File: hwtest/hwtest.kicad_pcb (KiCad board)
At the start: 2 copper layers, 103.3 x 65 mm, 299 parts, among them P1 RZM001P02T2L, P10 RZM001P02T2L, P11 RZM001P02T2L, P12 RZM001P02T2L, P13 RZM001P02T2L, P14 RZM001P02T2L, P15 RZM001P02T2L, P16 RZM001P02T2L, P17 RZM001P02T2L, P18 RZM001P02T2L, P19 RZM001P02T2L, P2 RZM001P02T2L, P20 RZM001P02T2L, P21 RZM001P02T2L, P22 RZM001P02T2L, P23 RZM001P02T2L, P24 RZM001P02T2L, P25 RZM001P02T2L, P26 RZM001P02T2L, P27 RZM001P02T2L, P28 RZM001P02T2L, P29 RZM001P02T2L, P3 RZM001P02T2L, P30 RZM001P02T2L, P31 RZM001P02T2L, P32 RZM001P02T2L, P33 RZM001P02T2L, P34 RZM001P02T2L, P35 RZM001P02T2L, P36 RZM001P02T2L, P37 RZM001P02T2L, P38 RZM001P02T2L, P39 RZM001P02T2L, P4 RZM001P02T2L, P40 RZM001P02T2L, P41 RZM001P02T2L, P42 RZM001P02T2L, P43 RZM001P02T2L, P44 RZM001P02T2L, P45 RZM001P02T2L, P46 RZM001P02T2L, P47 RZM001P02T2L, P48 RZM001P02T2L, P49 RZM001P02T2L, P5 RZM001P02T2L, P50 RZM001P02T2L, P51 RZM001P02T2L, P52 RZM001P02T2L, P53 RZM001P02T2L, P54 RZM001P02T2L, P55 RZM001P02T2L, P56 RZM001P02T2L, P57 RZM001P02T2L, P6 RZM001P02T2L, P7 RZM001P02T2L, P8 RZM001P02T2L, P9 RZM001P02T2L

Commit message: Tweak design.
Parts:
- N10, N11, N12, N13, N17, N18, N19, N28, N29, N9: value 2SK3541 -> NX7002BKMB315
- P10, P11, P12, P13, P17, P18, P19, P28, P29, P9: value RZM001P02T2L -> BSS84KNC
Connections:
- R30 pad 2: Net-(D13-A) -> GND
- R36 pad 2: Net-(D16-A) -> GND
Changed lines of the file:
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@@
 			)
 		)
-		(property "Value" "2SK3541"
+		(property "Value" "NX7002BKMB315"
 			(at 0 1.6 0)
 			(layer "User.3")
@@
 			(layers "F.Cu" "F.Mask" "F.Paste")
 			(roundrect_rratio 0.25)
-			(net 114 "Net-(D16-A)")
+			(net 4 "GND")
 			(pintype "passive")
 		)
@@
 			)
 		)
-		(property "Value" "RZM001P02T2L"
+		(property "Value" "BSS84KNC"
 			(at 0 1.6 0)
 			(layer "User.3")
@@
 			)
 		)
-		(property "Value" "2SK3541"
+		(property "Value" "NX7002BKMB315"
 			(at 0 1.6 0)
 			(layer "User.3")
@@
 			)
 		)
-		(property "Value" "2SK3541"
+		(property "Value" "NX7002BKMB315"
 			(at 0 1.6 0)
 			(layer "User.3")
@@
 			)
 		)
-		(property "Value" "2SK3541"
+		(property "Value" "NX7002BKMB315"
 			(at 0 1.6 0)
 			(layer "User.3")
@@
 			)
 		)
-		(property "Value" "2SK3541"
+		(property "Value" "NX7002BKMB315"
 			(at 0 1.6 0)
 			(layer "User.3")
@@
 			)
 		)
-		(property "Value" "2SK3541"
+		(property "Value" "NX7002BKMB315"
 			(at 0 1.6 0)
 			(layer "User.3")
@@
 			)
 		)
-		(property "Value" "RZM001P02T2L"
+		(property "Value" "BSS84KNC"
 			(at 0 1.6 0)
 			(layer "User.3")
@@
 			)
 		)
-		(property "Value" "2SK3541"
+		(property "Value" "NX7002BKMB315"
 			(at 0 1.6 0)
 			(layer "User.3")
@@
 			)
 		)
-		(property "Value" "RZM001P02T2L"
+		(property "Value" "BSS84KNC"
 			(at 0 1.6 0)
 			(layer "User.3")
@@
 			)
 		)
-		(property "Value" "2SK3541"
+		(property "Value" "NX7002BKMB315"
 			(at 0 1.6 0)
 			(layer "User.3")
@@
 			(layers "F.Cu" "F.Mask" "F.Paste")
 			(roundrect_rratio 0.25)
-			(net 111 "Net-(D13-A)")
+			(net 4 "GND")
 			(pintype "passive")
 		)
@@
 			)
 		)
-		(property "Value" "RZM001P02T2L"
+		(property "Value" "BSS84KNC"
 			(at 0 1.6 0)
 			(layer "User.3")
@@
 			)
 		)
-		(property "Value" "2SK3541"
+		(property "Value" "NX7002BKMB315"
 			(at 0 1.6 0)
 			(layer "User.3")
@@
 			)
 		)
-		(property "Value" "RZM001P02T2L"
+		(property "Value" "BSS84KNC"
 			(at 0 1.6 0)
 			(layer "User.3")
@@
 			)
 		)
-		(property "Value" "RZM001P02T2L"
+		(property "Value" "BSS84KNC"
 			(at 0 1.6 0)
 			(layer "User.3")
@@
 			)
 		)
-		(property "Value" "RZM001P02T2L"
+		(property "Value" "BSS84KNC"
 			(at 0 1.6 0)
 			(layer "User.3")
@@
 			)
 		)
-		(property "Value" "RZM001P02T2L"
+		(property "Value" "BSS84KNC"
 			(at 0 1.6 0)
 			(layer "User.3")
@@
 			)
 		)
-		(property "Value" "RZM001P02T2L"
+		(property "Value" "BSS84KNC"
 			(at 0 1.6 0)
 			(layer "User.3")
@@
 			)
 		)
-		(property "Value" "RZM001P02T2L"
+		(property "Value" "BSS84KNC"
 			(at 0 1.6 0)
 			(layer "User.3")
@@
 			)
 		)
-		(property "Value" "2SK3541"
+		(property "Value" "NX7002BKMB315"
 			(at 0 1.6 0)
 			(layer "User.3")

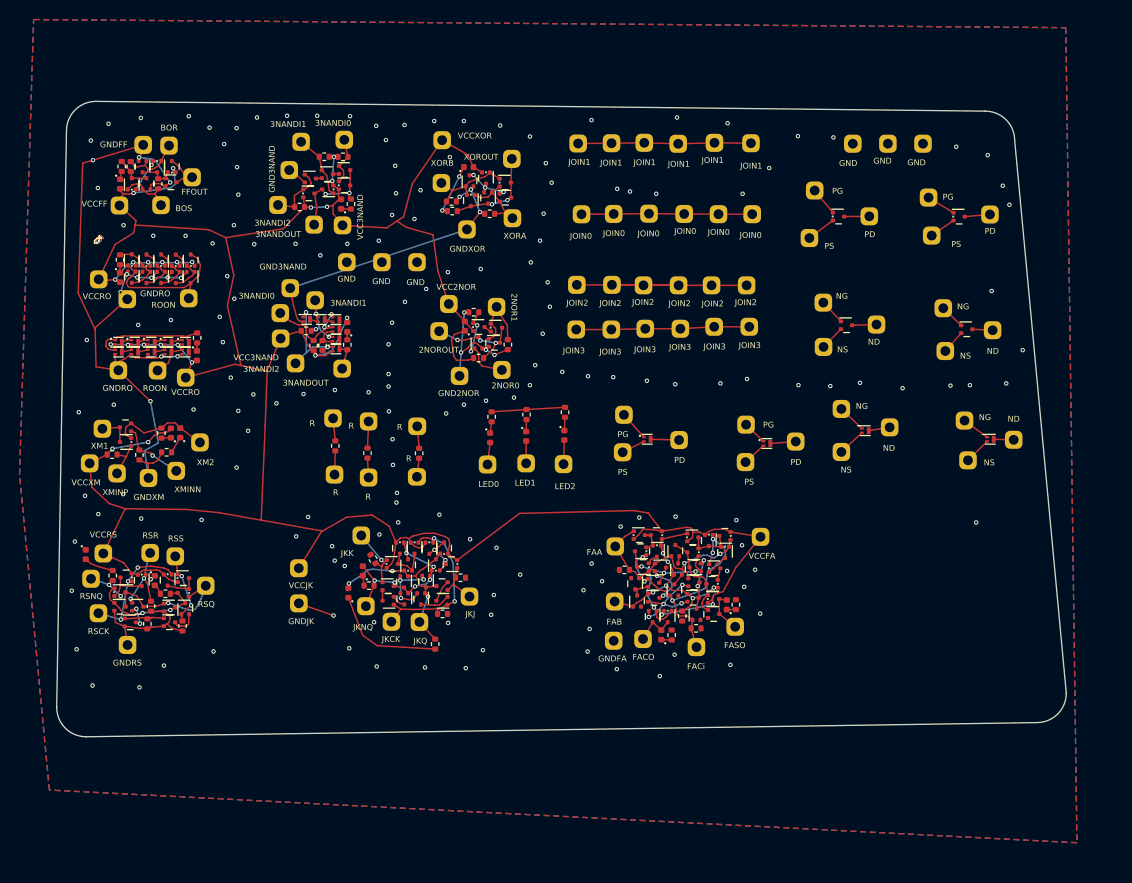
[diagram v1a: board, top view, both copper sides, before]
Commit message: bump for order version
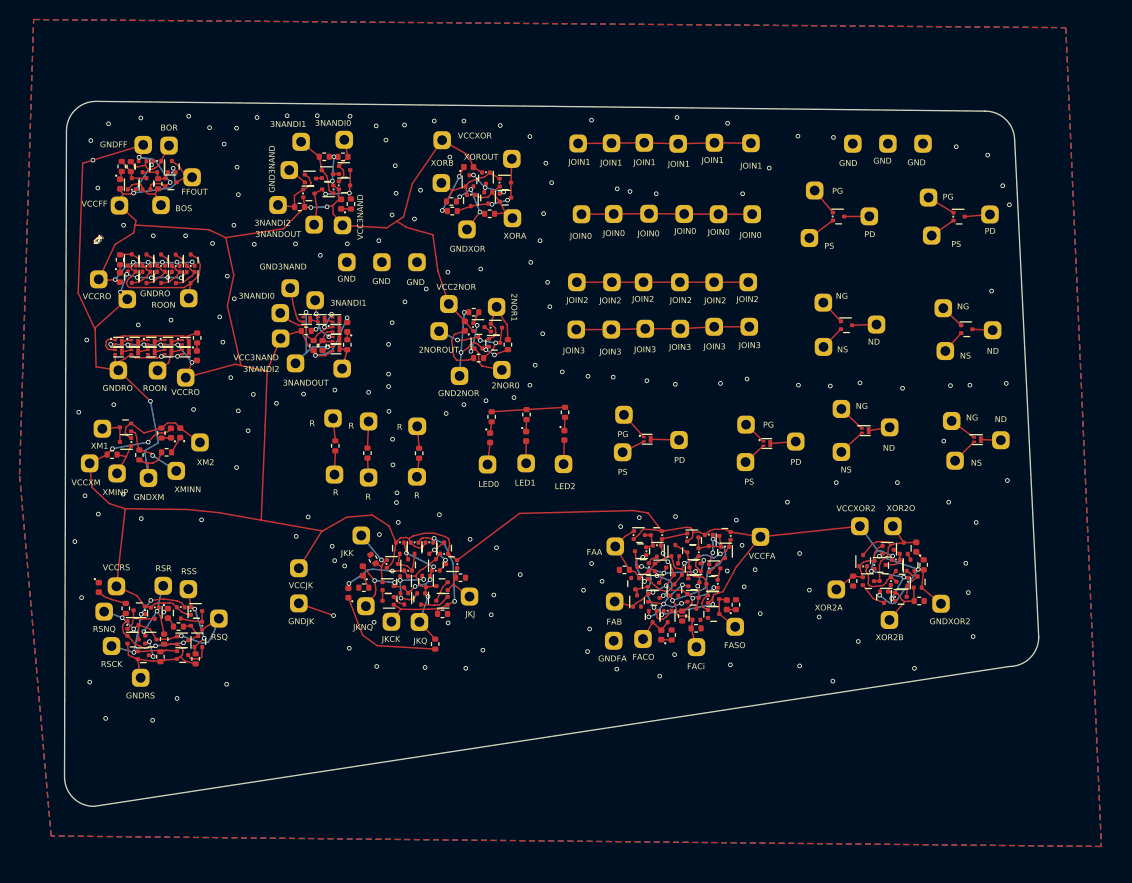
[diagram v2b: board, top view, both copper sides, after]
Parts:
- added D19: LED, cnhardware:LED_0402_1005Metric_COMPACT, F.Cu at (117.9, 63.6)
- added N58: 2SK3541, cnhardware:SOT-723-COMPACT, F.Cu at (116.7, 63.7)
- added N59: 2SK3541, cnhardware:SOT-723-COMPACT, F.Cu at (113.0, 67.1)
- added N60: 2SK3541, cnhardware:SOT-723-COMPACT, F.Cu at (117.3, 65.5)
- added N61: 2SK3541, cnhardware:SOT-723-COMPACT, F.Cu at (114.6, 68.7)
- added N62: 2SK3541, cnhardware:SOT-723-COMPACT, F.Cu at (115.1, 63.9)
- added N63: 2SK3541, cnhardware:SOT-723-COMPACT, F.Cu at (118.1, 67.2)
- added P58: RZM001P02T2L, cnhardware:SOT-723-COMPACTP, F.Cu at (115.8, 65.5)
- added P59: RZM001P02T2L, cnhardware:SOT-723-COMPACTP, F.Cu at (116.5, 67.1)
- added P60: RZM001P02T2L, cnhardware:SOT-723-COMPACTP, F.Cu at (114.8, 67.1)
- added P61: RZM001P02T2L, cnhardware:SOT-723-COMPACTP, F.Cu at (112.5, 65.0)
- added P62: RZM001P02T2L, cnhardware:SOT-723-COMPACTP, F.Cu at (114.2, 65.4)
- added P63: RZM001P02T2L, cnhardware:SOT-723-COMPACTP, F.Cu at (116.4, 68.7)
- added R45: 1k, cnhardware:R_0402_1005Metric_COMPACT, F.Cu at (118.7, 65.4)
- added R46: 1k, cnhardware:R_0402_1005Metric_COMPACT, F.Cu at (118.2, 69.1)
- added R47: 1k, cnhardware:R_0402_1005Metric_COMPACT, F.Cu at (111.5, 67.1)
- added TP124: XOR2A, cnhardware:TPTHRU, F.Cu at (109.8, 67.9)
- added TP125: XOR2B, cnhardware:TPTHRU, F.Cu at (115.2, 71.1)
- added TP126: XOR2O, cnhardware:TPTHRU, F.Cu at (115.5, 61.5)
- added TP127: VCCXOR2, cnhardware:TPTHRU, F.Cu at (112.2, 61.5)
- added TP128: GNDXOR2, cnhardware:TPTHRU, F.Cu at (120.5, 69.4)
- moved D14 3.62 mm to (34.3, 67.7)
- moved D15 3.62 mm to (41.4, 70.4)
- moved N35 3.62 mm to (39.6, 73.1)
- moved N36 3.62 mm to (38.9, 74.7)
- moved N38 3.62 mm to (42.9, 73.1)
- moved N39 3.62 mm to (44.5, 73.2)
- moved N40 3.62 mm to (42.9, 74.6)
- moved R31 3.62 mm to (37.1, 69.9)
- moved R32 3.62 mm to (42.5, 71.7)
- moved R33 3.62 mm to (44.2, 75.0)
- moved R34 3.62 mm to (41.0, 73.0)
- moved TP106 3.62 mm to (34.9, 70.2)
- moved TP107 3.62 mm to (46.6, 70.9)
- moved TP111 3.62 mm to (38.6, 77.0)
- moved N37 3.62 mm to (37.8, 73.1)
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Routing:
- net VDD: track 306.1 -> 333.8 mm, vias 25 -> 29
- net Net-(D19-A): track 0.00 -> 12.9 mm
- net Net-(TP85-Pad1): track 27.8 -> 17.5 mm
- net Net-(N59-G): track 0.00 -> 8.07 mm
- net Net-(N61-G): track 0.00 -> 7.65 mm
- net Net-(P58-D): track 0.00 -> 6.21 mm
- net Net-(N60-G): track 0.00 -> 3.82 mm
- net Net-(N58-G): track 0.00 -> 3.05 mm
- net Net-(N59-S): track 0.00 -> 2.93 mm
- net GND: track 168.9 -> 166.3 mm, vias 192 -> 210
- net Net-(D19-K): track 0.00 -> 1.11 mm
- net Net-(N58-S): track 0.00 -> 0.66 mm
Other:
- board size 103.3 x 65 mm -> 99.7 x 72.1 mm

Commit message: Tweak test
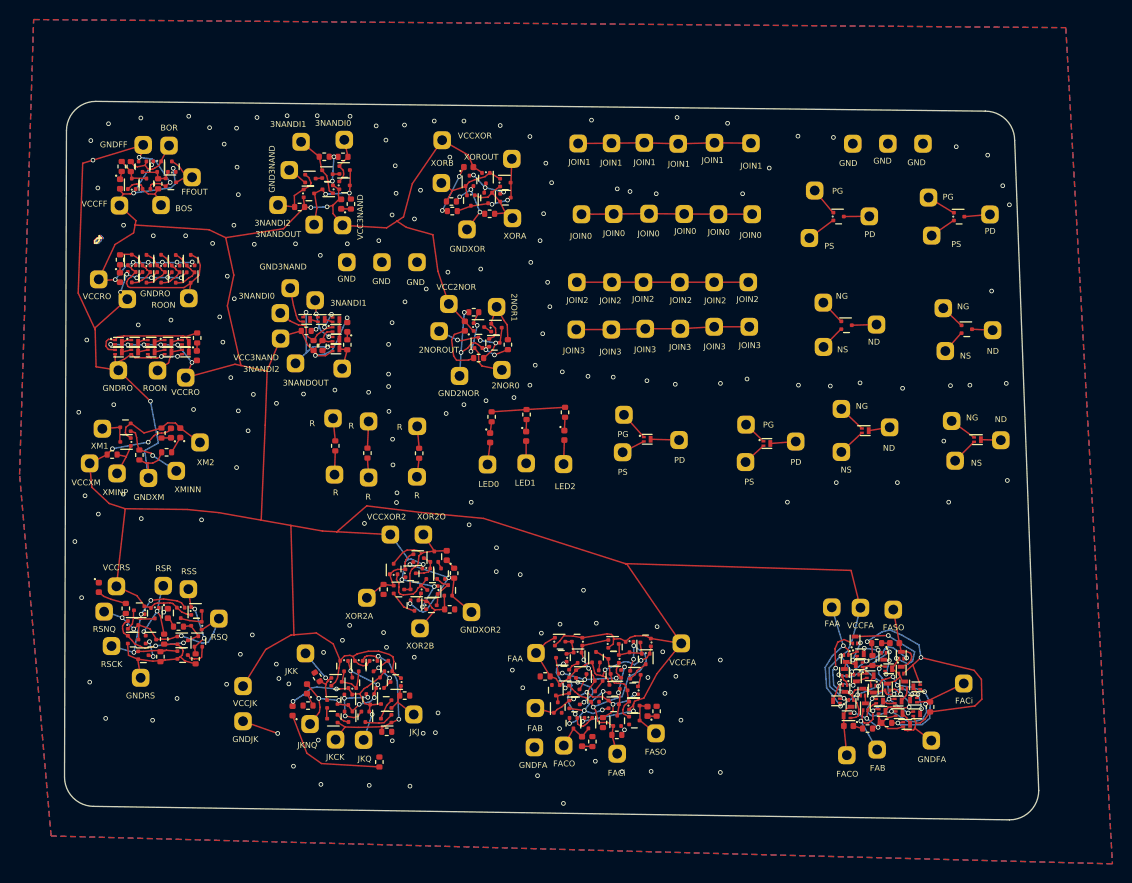
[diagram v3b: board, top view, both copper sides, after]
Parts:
- added D20: LED, cnhardware:LED_0402_1005Metric_COMPACT, F.Cu at (111.0, 81.9)
- added D21: LED, cnhardware:LED_0402_1005Metric_COMPACT, F.Cu at (115.7, 73.4)
- added N64: 2SK3541, cnhardware:DFN1006-3-NCH, F.Cu at (118.0, 80.7)
- added N65: 2SK3541, cnhardware:DFN1006-3-NCH, F.Cu at (117.7, 79.2)
- added N66: 2SK3541, cnhardware:DFN1006-3-NCH, F.Cu at (118.0, 77.9)
- added N67: 2SK3541, cnhardware:DFN1006-3-NCH, F.Cu at (110.9, 80.8)
- added N68: 2SK3541, cnhardware:DFN1006-3-NCH, F.Cu at (112.5, 78.4)
- added N69: 2SK3541, cnhardware:DFN1006-3-NCH, F.Cu at (112.7, 79.9)
- added N70: 2SK3541, cnhardware:DFN1006-3-NCH, F.Cu at (116.8, 77.7)
- added N71: 2SK3541, cnhardware:DFN1006-3-NCH, F.Cu at (116.1, 79.3)
- added N72: 2SK3541, cnhardware:DFN1006-3-NCH, F.Cu at (114.2, 79.4)
- added N73: 2SK3541, cnhardware:DFN1006-3-NCH, F.Cu at (117.0, 81.7)
- added N74: 2SK3541, cnhardware:DFN1006-3-NCH, F.Cu at (115.0, 77.9)
- added N75: 2SK3541, cnhardware:DFN1006-3-NCH, F.Cu at (114.4, 80.4)
- added N76: 2SK3541, cnhardware:DFN1006-3-NCH, F.Cu at (116.4, 76.2)
- added N77: 2SK3541, cnhardware:DFN1006-3-NCH, F.Cu at (116.2, 80.6)
- added P64: RZM001P02T2L, cnhardware:DFN1006-3-PCH, F.Cu at (109.8, 79.3)
- added P65: RZM001P02T2L, cnhardware:DFN1006-3-PCH, F.Cu at (113.2, 76.8)
- added P66: RZM001P02T2L, cnhardware:DFN1006-3-PCH, F.Cu at (113.5, 78.1)
- added P67: RZM001P02T2L, cnhardware:DFN1006-3-PCH, F.Cu at (111.3, 79.6)
- added P68: RZM001P02T2L, cnhardware:DFN1006-3-PCH, F.Cu at (111.8, 77.0)
- added P69: RZM001P02T2L, cnhardware:DFN1006-3-PCH, F.Cu at (110.6, 78.1)
- added P70: RZM001P02T2L, cnhardware:DFN1006-3-PCH, F.Cu at (110.6, 76.4)
- added P71: RZM001P02T2L, cnhardware:DFN1006-3-PCH, F.Cu at (111.7, 73.1)
- added P72: RZM001P02T2L, cnhardware:DFN1006-3-PCH, F.Cu at (110.8, 75.0)
- added P73: RZM001P02T2L, cnhardware:DFN1006-3-PCH, F.Cu at (112.2, 74.5)
- added P74: RZM001P02T2L, cnhardware:DFN1006-3-PCH, F.Cu at (114.6, 74.8)
- added P75: RZM001P02T2L, cnhardware:DFN1006-3-PCH, F.Cu at (115.1, 76.0)
- added P76: RZM001P02T2L, cnhardware:DFN1006-3-PCH, F.Cu at (112.1, 75.6)
- added P77: RZM001P02T2L, cnhardware:DFN1006-3-PCH, F.Cu at (116.4, 74.7)
- added R48: 1k, cnhardware:R_0402_1005Metric_COMPACT, F.Cu at (119.3, 80.0)
- added R49: 1k, cnhardware:R_0402_1005Metric_COMPACT, F.Cu at (113.5, 75.2)
- added R50: 1k, cnhardware:R_0402_1005Metric_COMPACT, F.Cu at (114.9, 81.6)
- added R51: 1k, cnhardware:R_0402_1005Metric_COMPACT, F.Cu at (113.0, 82.2)
- added R52: 1k, cnhardware:R_0402_1005Metric_COMPACT, F.Cu at (113.9, 73.4)
- added TP129: FACi, cnhardware:TPTHRU, F.Cu at (122.8, 77.5)
- added TP130: FAB, cnhardware:TPTHRU, F.Cu at (113.9, 84.3)
- added TP131: FAA, cnhardware:TPTHRU, F.Cu at (109.3, 69.8)
- added TP132: FACO, cnhardware:TPTHRU, F.Cu at (110.8, 84.9)
- added TP133: FASO, cnhardware:TPTHRU, F.Cu at (115.6, 70.0)
- added TP134: VCCFA, cnhardware:TPTHRU, F.Cu at (112.2, 69.8)
- added TP135: GNDFA, cnhardware:TPTHRU, F.Cu at (119.5, 83.4)
- moved D19 48.0 mm to (69.9, 64.5)
- moved N58 48.0 mm to (68.6, 64.6)
- moved N59 48.0 mm to (65.0, 67.9)
- moved N60 48.0 mm to (69.3, 66.3)
- moved N61 48.0 mm to (66.6, 69.6)
- moved N62 48.0 mm to (67.0, 64.7)
- moved N63 48.0 mm to (70.0, 68.0)
- moved P58 48.0 mm to (67.8, 66.3)
- moved P59 48.0 mm to (68.4, 68.0)
- moved P60 48.0 mm to (66.7, 67.9)
- moved P61 48.0 mm to (64.5, 65.8)
- moved P62 48.0 mm to (66.2, 66.3)
- moved P63 48.0 mm to (68.3, 69.5)
- moved R45 48.0 mm to (70.7, 66.3)
- moved R46 48.0 mm to (70.2, 70.0)
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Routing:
- net VDD: track 333.8 -> 409.6 mm, vias 29 -> 34
- net GND: track 166.3 -> 214.0 mm, vias 210 -> 213
- net FAAs: track 0.00 -> 33.7 mm, vias 0 -> 8
- net FACis: track 0.00 -> 28.1 mm, vias 0 -> 5
- net FABs: track 0.00 -> 20.8 mm, vias 0 -> 5
- net Xs: track 0.00 -> 20.3 mm, vias 0 -> 4
- net Net-(N70-D): track 0.00 -> 14.4 mm, vias 0 -> 2
- net Net-(N73-D): track 0.00 -> 7.60 mm, vias 0 -> 2
- net SOUTs: track 0.00 -> 7.36 mm
- net Net-(P70-D): track 0.00 -> 5.51 mm, vias 0 -> 2
- net Net-(P64-D): track 0.00 -> 5.36 mm, vias 0 -> 2
- net COUTs: track 0.00 -> 5.34 mm
- net Net-(N64-D): track 0.00 -> 3.30 mm, vias 0 -> 2
- net Net-(P73-D): track 0.00 -> 2.46 mm, vias 0 -> 2
- net Net-(D16-A): track 20.5 -> 18.1 mm
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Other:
- board size 99.7 x 72.1 mm -> 99.7 x 73.5 mm
